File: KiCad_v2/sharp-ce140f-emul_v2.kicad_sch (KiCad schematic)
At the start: 50 parts, among them J1 ext pins, J2 Sharp PC 11-pin, J3 USB_B_Micro, J4 Micro_SD_Card_Det, J5 Battery, J6 SWD, SW1 AYZ0102AGRLC, U1 TXS0108EPW, U2 STM32L432KCUx, U4 MCP73831, U5 XC6206P332MR, Y1 32.768KHz

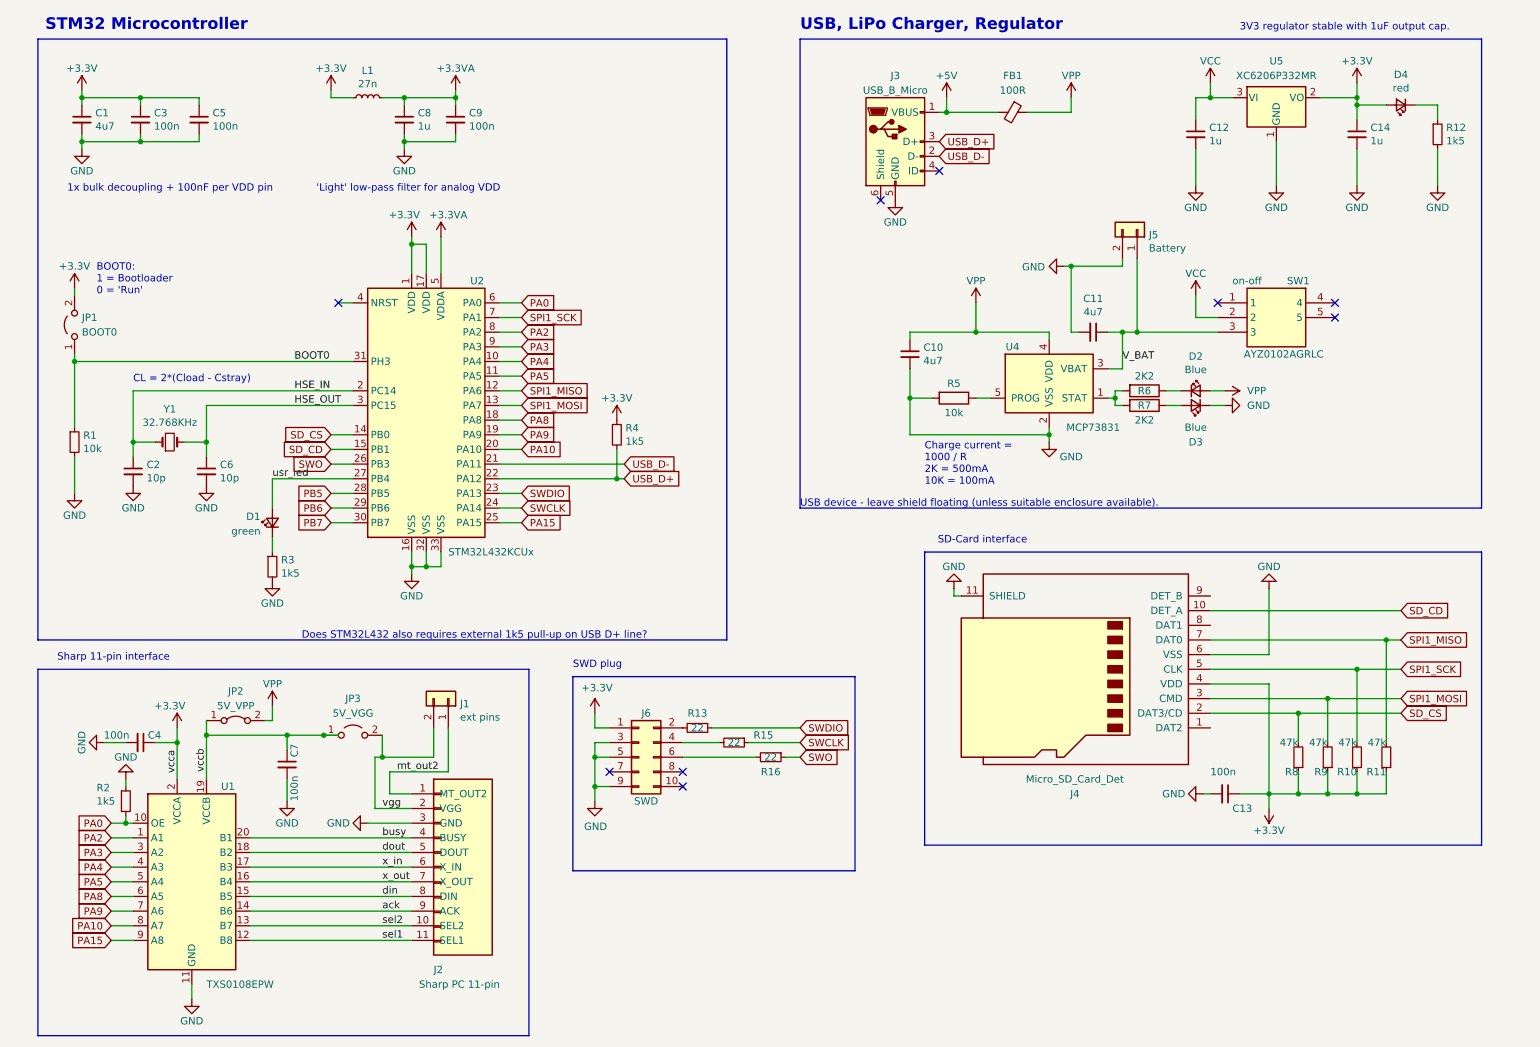
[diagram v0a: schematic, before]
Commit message: DRAFT v2 schematics revisions
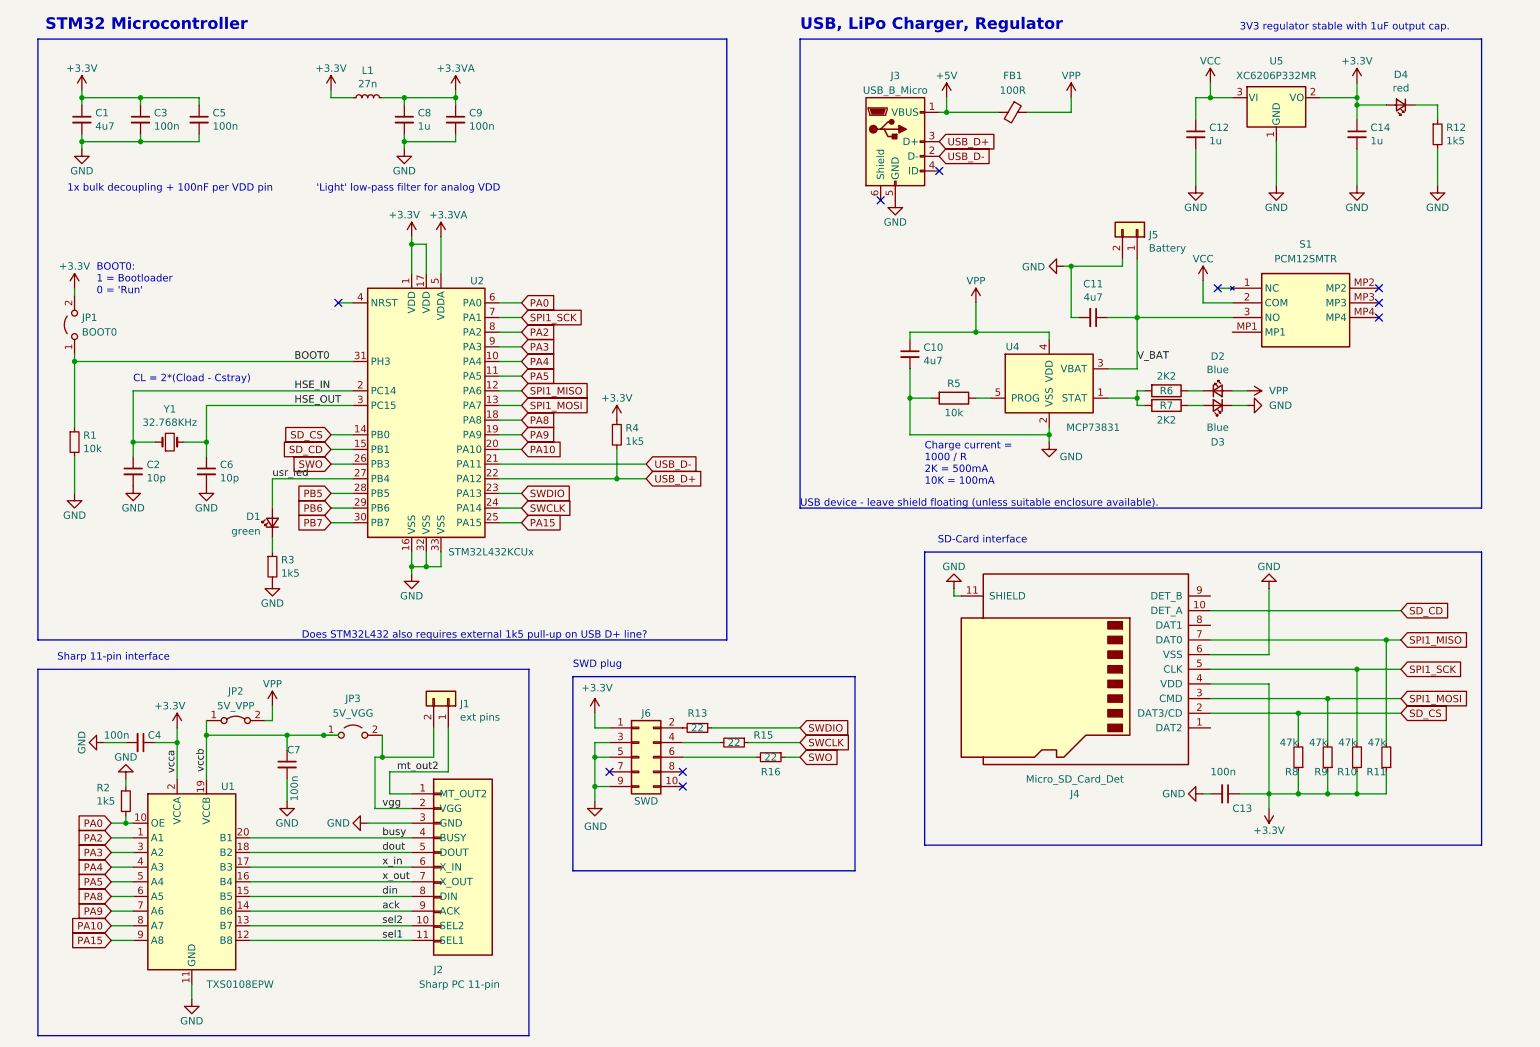
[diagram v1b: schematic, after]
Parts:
- removed SW1: AYZ0102AGRLC, SamacSys_Parts:AYZ0102AGRLC, symbol SamacSys_Parts:AYZ0102AGRLC
- added S1: PCM12SMTR, ce140f_library:PCM12SMTR, symbol ce140f_Library:PCM12SMTR
- C1, C10, C11, C12, C14: footprint Capacitor_SMD:C_0603_1608Metric -> ce140f_library:C_0603_1608Metric
- C13, C2, C3, C4, C5, C6, C7, C8, C9: footprint Capacitor_SMD:C_0402_1005Metric -> ce140f_library:C_0603_1608Metric
- L1: footprint Inductor_SMD:L_0402_1005Metric -> Inductor_SMD:L_0603_1608Metric
- R1, R10, R11, R13, R15, R16, R2, R4, R8, R9: footprint Resistor_SMD:R_0402_1005Metric -> ce140f_library:R_0603_1608Metric
- R12, R3, R5, R6, R7: footprint Resistor_SMD:R_0603_1608Metric -> ce140f_library:R_0603_1608Metric
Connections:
- net VCC: now also S1.2 (COM)
- net V_BAT: now also S1.3 (NO)
- no-connect marks 9 -> 10
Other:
- moved on the sheet: C11, D2, D3, R6, R7
